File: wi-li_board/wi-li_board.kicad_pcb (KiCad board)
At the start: 2 copper layers, 20.8 x 79.6 mm, 30 parts, among them J1 Barrel_Jack_MountingPin, J2 2059-302/998-403, J3 2059-302/998-403, J4 2059-302/998-403, Q1 Q_NMOS_DGS, Q2 Q_NMOS_DGS, Q3 Q_NMOS_DGS, U1 AP1509, U2 ESP-12E

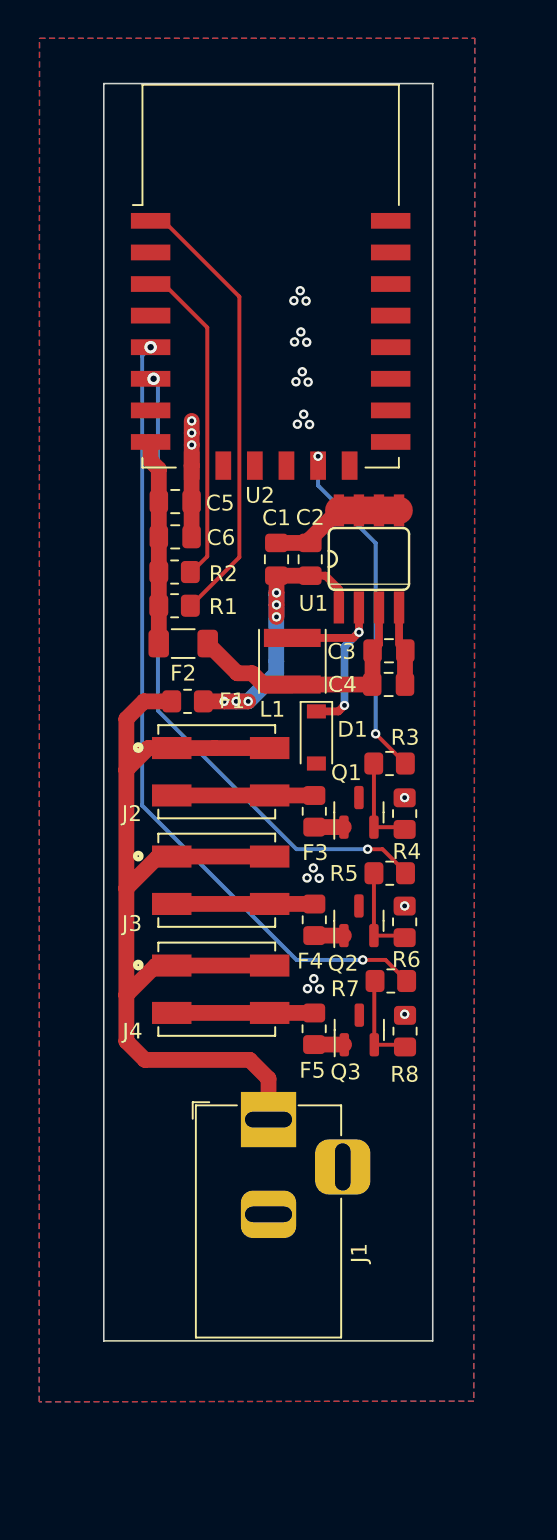
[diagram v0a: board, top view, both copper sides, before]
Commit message: fix issues from first rev
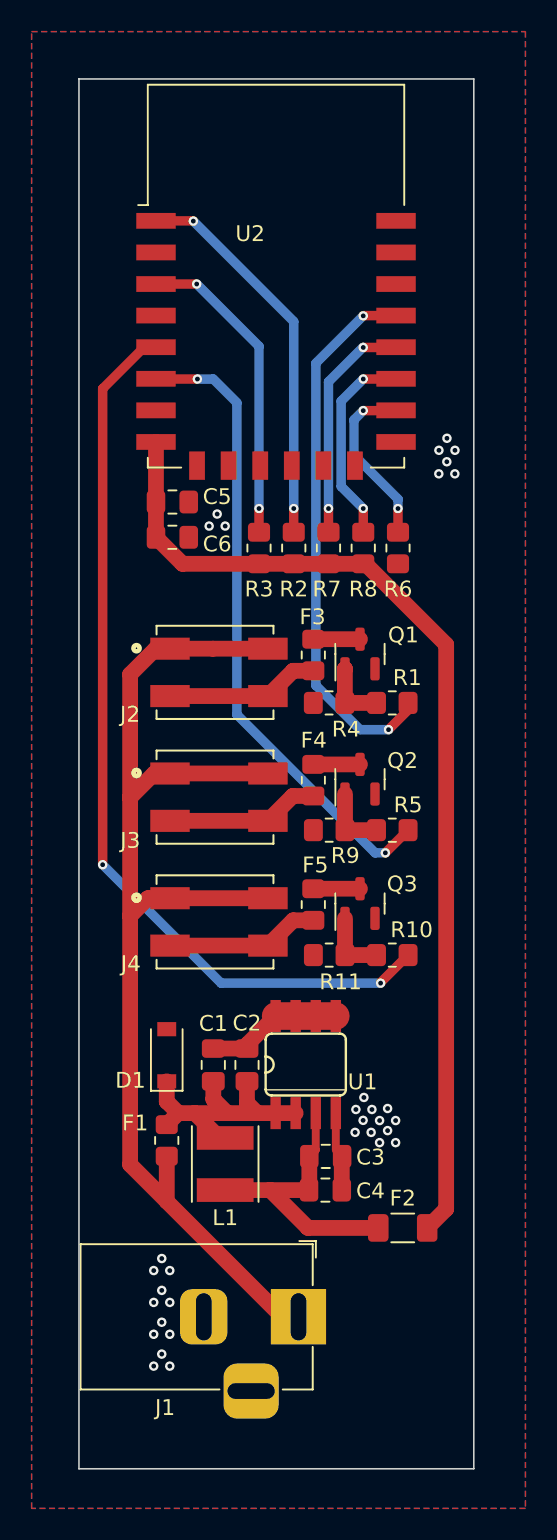
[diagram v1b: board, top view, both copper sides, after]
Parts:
- added R10: 330, Resistor_SMD:R_0805_2012Metric_Pad1.20x1.40mm_HandSolder, F.Cu at (149.8, 105.5)
- added R11: 10k, Resistor_SMD:R_0805_2012Metric_Pad1.20x1.40mm_HandSolder, F.Cu at (145.8, 105.5)
- added R9: 10k, Resistor_SMD:R_0805_2012Metric_Pad1.20x1.40mm_HandSolder, F.Cu at (145.8, 97.6)
- L1: footprint Inductor_SMD:L_Vishay_IFSC-1515AH_4x4x1.8mm -> RLC:L_Vishay_IFSC-1515AH_HandSolder
- R1: value 10k -> 330
- R3, R7: value 330 -> 10k
- moved F2 39.5 mm to (150.5, 122.8), turned to 180 degrees
- moved C1 32.3 mm to (138.5, 112.4)
- moved C2 32.3 mm to (140.6, 112.4)
- moved C3 32.3 mm to (145.6, 118.2)
- moved C4 32.3 mm to (145.6, 120.4)
- moved U1 32.3 mm to (144.4, 112.4)
- moved L1 32.1 mm to (139.3, 118.7)
- moved R8 30.7 mm to (148.0, 79.7), turned to 90 degrees
- moved F1 27.8 mm to (135.6, 117.2), turned to -90 degrees
- moved R7 27.7 mm to (145.8, 79.7), turned to 90 degrees
- moved R6 23.7 mm to (150.2, 79.7), turned to 90 degrees
- moved D1 22.2 mm to (135.6, 111.8), turned to 90 degrees
- moved R3 16.0 mm to (141.4, 79.7), turned to 90 degrees
- moved R1 15.1 mm to (149.8, 89.5)
- moved J1 12.6 mm to (143.9, 128.4), turned to 0 degrees
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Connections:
- C1 pad 2: Net-(C1-Pad2) -> Net-(D1-Pad1)
- C2 pad 1: Net-(C1-Pad2) -> Net-(D1-Pad1)
- F1 pad 1: Net-(C1-Pad2) -> Net-(D1-Pad1)
- Q1 pad 1: Net-(F3-Pad1) -> Net-(Q1-Pad1)
- Q1 pad 2: Net-(Q1-Pad2) -> GND
- Q1 pad 3: GND -> Net-(F3-Pad1)
- Q2 pad 1: Net-(F4-Pad1) -> Net-(Q2-Pad1)
- Q2 pad 2: Net-(Q2-Pad2) -> GND
- Q2 pad 3: GND -> Net-(F4-Pad1)
- Q3 pad 1: Net-(F5-Pad1) -> Net-(Q3-Pad1)
- Q3 pad 2: Net-(Q3-Pad2) -> GND
- Q3 pad 3: GND -> Net-(F5-Pad1)
- R1 pad 1: VDD -> Net-(Q1-Pad1)
- R1 pad 2: Net-(R1-Pad2) -> GPIO_4
- R3 pad 1: Net-(Q1-Pad2) -> VDD
- R3 pad 2: GPIO_4 -> Net-(R3-Pad2)
- R4 pad 2: Net-(Q1-Pad2) -> Net-(Q1-Pad1)
- R5 pad 1: Net-(Q2-Pad2) -> Net-(Q2-Pad1)
- R6 pad 2: Net-(Q2-Pad2) -> Net-(R6-Pad2)
- R7 pad 1: Net-(Q3-Pad2) -> VDD
- R7 pad 2: GPIO_14 -> Net-(R7-Pad2)
- R8 pad 1: GND -> VDD
- R8 pad 2: Net-(Q3-Pad2) -> Net-(R8-Pad2)
- U1 pad 1: Net-(C1-Pad2) -> Net-(D1-Pad1)
- U2 pad 1: Net-(R1-Pad2) -> Net-(R2-Pad2)
- U2 pad 13: GPIO_4 -> unconnected-(U2-Pad13)
- U2 pad 14: GPIO_5 -> unconnected-(U2-Pad14)
- U2 pad 15: GPIO_3 -> GND
- U2 pad 16: unconnected-(U2-Pad16) -> Net-(R6-Pad2)
- U2 pad 17: unconnected-(U2-Pad17) -> Net-(R8-Pad2)
- U2 pad 18: unconnected-(U2-Pad18) -> Net-(R7-Pad2)
- U2 pad 19: GPIO9 -> GPIO_4
- U2 pad 20: GPIO10 -> unconnected-(U2-Pad20)
- U2 pad 3: Net-(R2-Pad2) -> Net-(R3-Pad2)
- U2 pad 4: GPIO_16 -> unconnected-(U2-Pad4)
- U2 pad 7: GPIO_13 -> unconnected-(U2-Pad7)
- U2 pad 9: GND -> unconnected-(U2-Pad9)
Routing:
- net VDD: track 13.0 -> 64.7 mm
- net Net-(R1-Pad2): track 28.5 -> 0.00 mm
- net Net-(C1-Pad2): track 20.1 -> 0.00 mm, vias 6 -> 0
- net Net-(R3-Pad2): track 0.00 -> 19.9 mm, vias 0 -> 2
- net Net-(R7-Pad2): track 0.00 -> 14.7 mm, vias 0 -> 2
- net GPIO_4: track 21.7 -> 34.7 mm
- net Net-(R8-Pad2): track 0.00 -> 12.9 mm, vias 0 -> 2
- net Net-(R6-Pad2): track 0.00 -> 11.2 mm, vias 0 -> 2
- net VCC: track 65.7 -> 76.5 mm
- net GND: track 21.1 -> 13.8 mm, vias 24 -> 33
- net GPIO_14: track 50.6 -> 57.8 mm
- net Net-(Q3-Pad2): track 6.06 -> 0.00 mm
- net Net-(Q1-Pad2): track 6.04 -> 0.00 mm
- net Net-(Q2-Pad2): track 5.95 -> 0.00 mm
- net Net-(D1-Pad1): track 12.9 -> 18.0 mm, vias 2 -> 0
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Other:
- board size 20.8 x 79.6 mm -> 25 x 88 mm
